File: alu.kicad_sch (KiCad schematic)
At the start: 20 parts, among them SW1 SW_DIP_x08

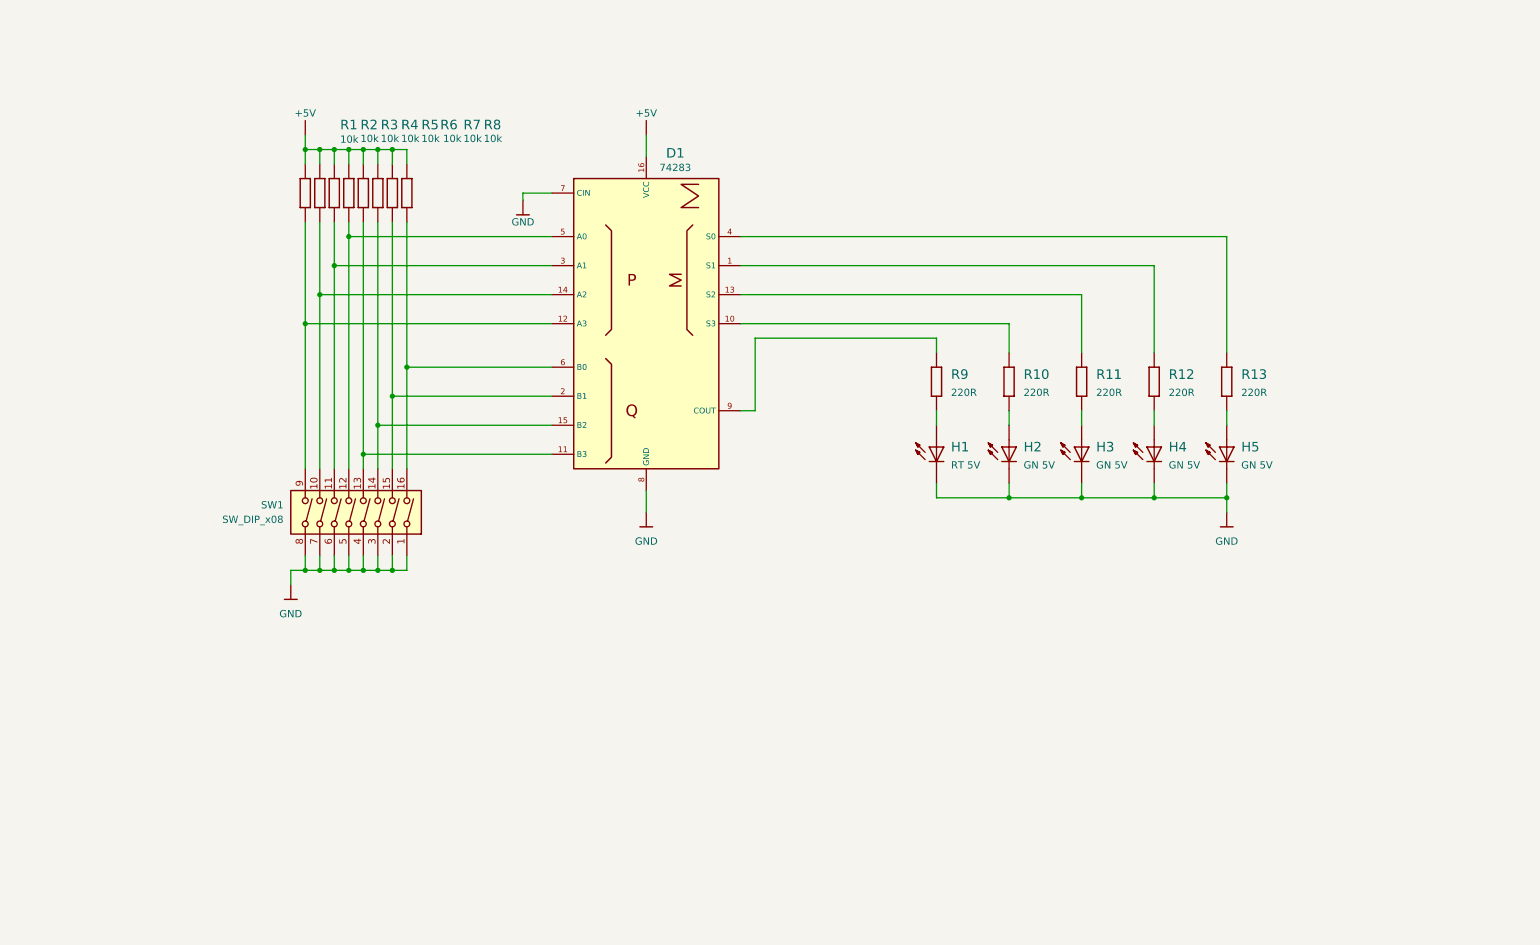
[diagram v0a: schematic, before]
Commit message: kys
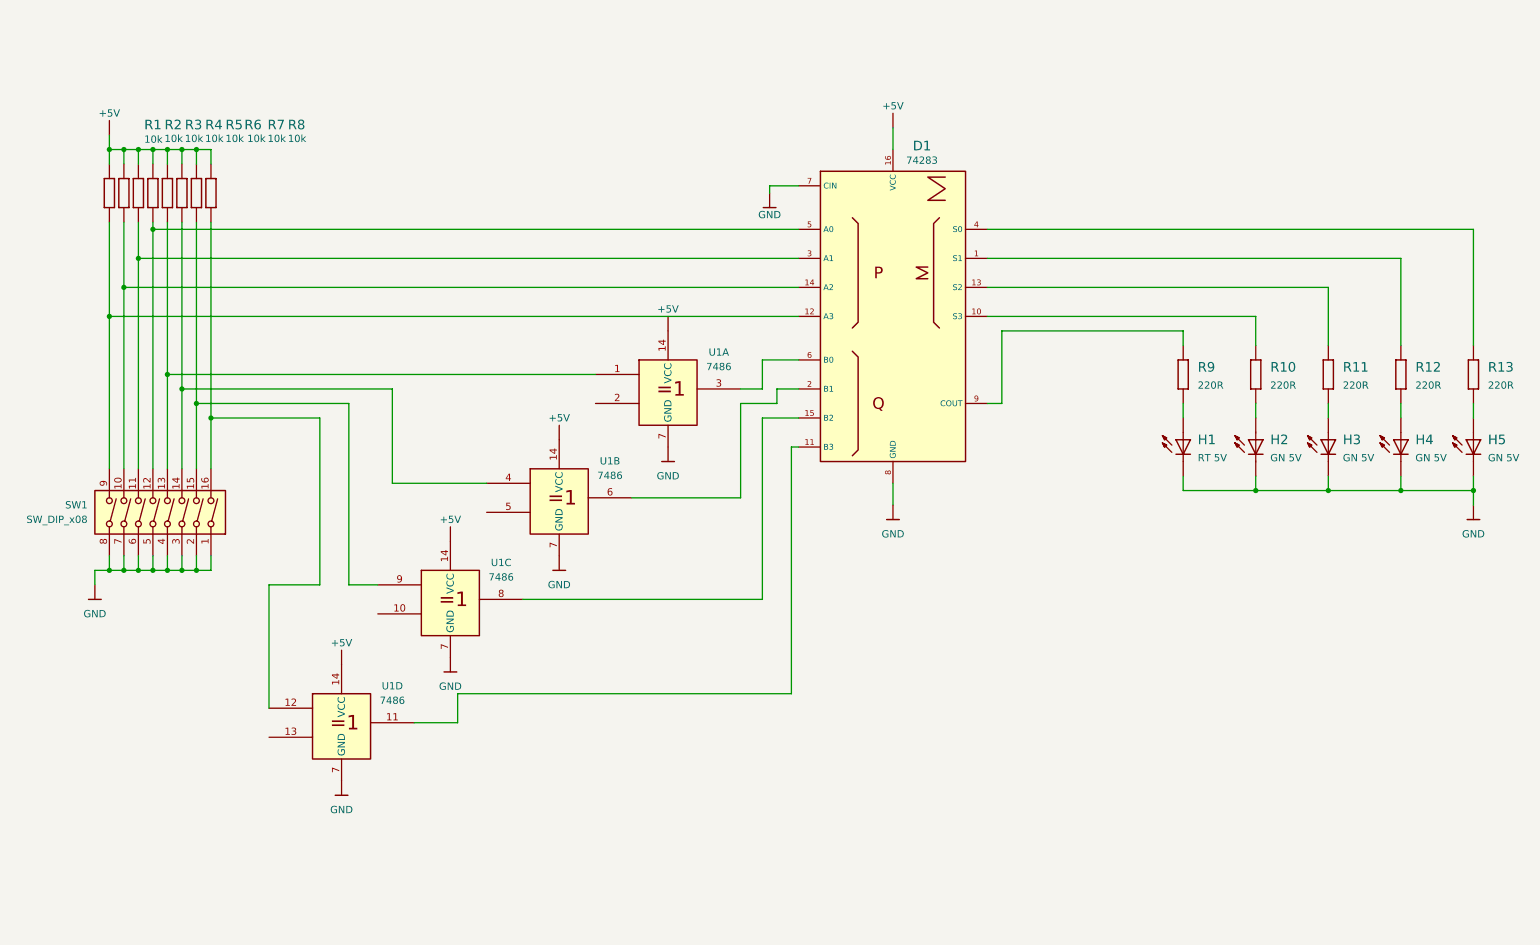
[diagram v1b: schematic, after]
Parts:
- added U1: 7486, symbol 74xx_IEEE:7486
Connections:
- net +5V: now also U1.14 (VCC), U1.14 (VCC), U1.14 (VCC), U1.14 (VCC)
- net GND: now also U1.7 (GND), U1.7 (GND), U1.7 (GND), U1.7 (GND)
- net at R5.1, SW1.13: now also U1.1; no longer D1.11 (B3)
- net at R6.1, SW1.14: now also U1.4; no longer D1.15 (B2)
- net at R7.1, SW1.15: now also U1.9; no longer D1.2 (B1)
- net at R8.1, SW1.16: now also U1.12; no longer D1.6 (B0)
- new net: D1.2 (B1), U1.6
- new net: D1.6 (B0), U1.3
- new net: D1.11 (B3), U1.11
- new net: D1.15 (B2), U1.8
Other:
- moved on the sheet: D1, H1, H2, H3, H4, H5, R1, R10, R11, R12, R13, R2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

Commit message: schem fixed
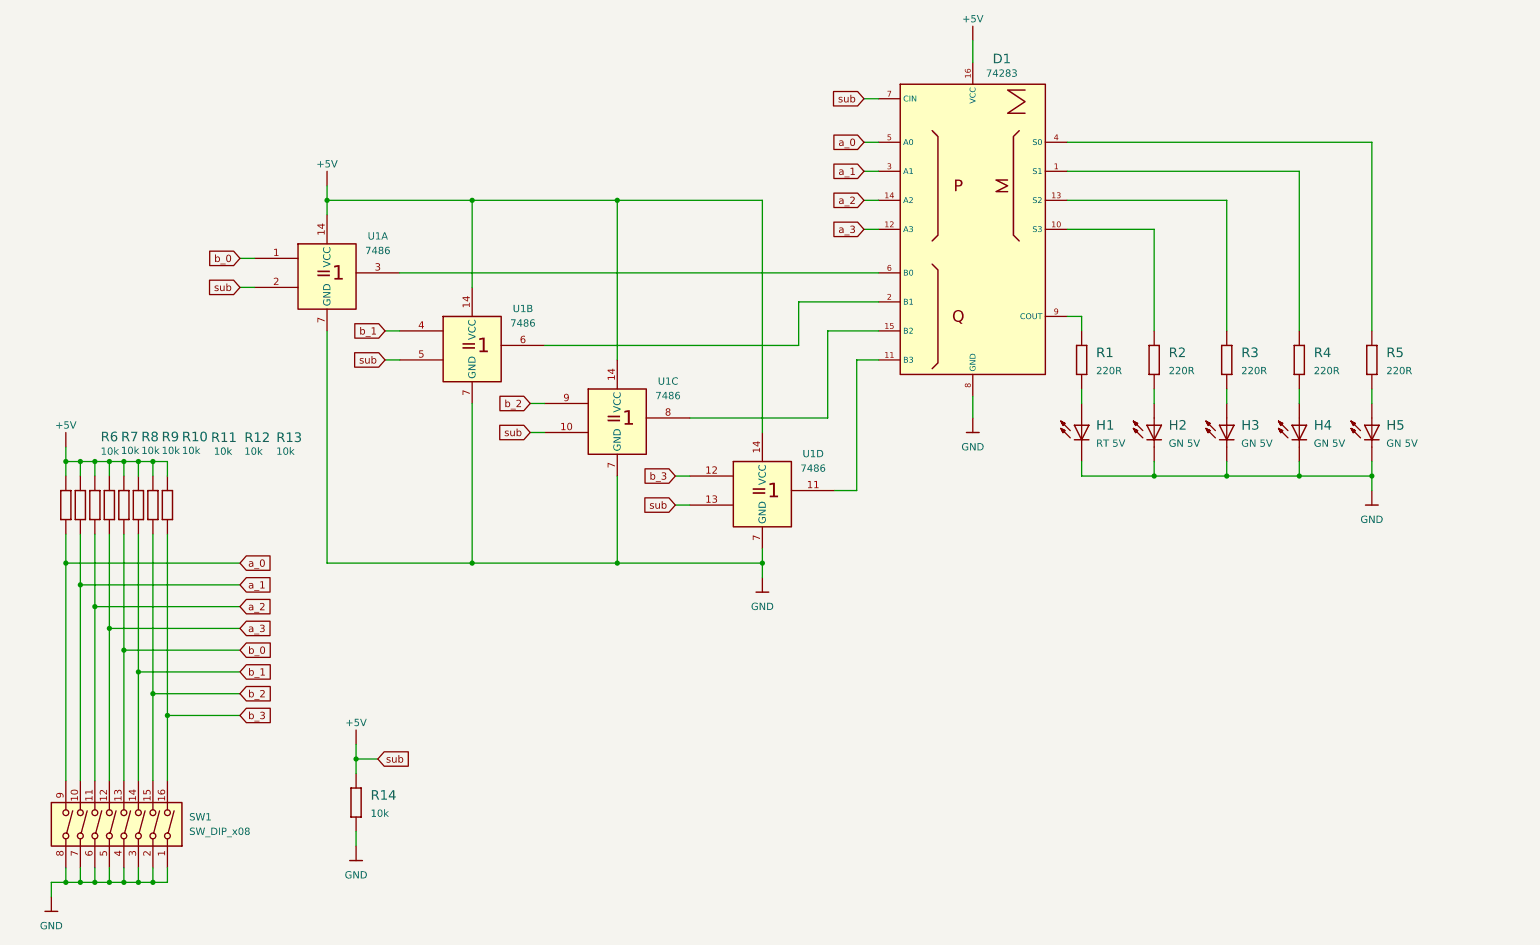
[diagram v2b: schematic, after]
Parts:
- added R14: 10k, ~footprint, symbol basic_AndF:R
- renumbered R9 to R1, R5 to R10, R6 to R11, R7 to R12, R8 to R13, R10 to R2, R11 to R3, R12 to R4, R13 to R5, R1 to R6, R2 to R7, R3 to R8, R4 to R9
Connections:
- net +5V: now also D1.7 (CIN), U1.10, U1.13, U1.2, U1.5, R14.2
- net GND: now also R14.1; no longer D1.7 (CIN)
- net a_1: now reaches R7.1, SW1.10
- net a_1: now also D1.3 (A1); no longer D1.14 (A2)
- net a_2: now reaches R8.1, SW1.11
- net a_2: now also D1.14 (A2); no longer D1.3 (A1)
- net a_3: now reaches R9.1, SW1.12
- net a_3: now also D1.12 (A3); no longer D1.5 (A0)
- net b_0: now reaches R10.1, SW1.13, U1.1
- net b_1: now reaches R11.1, SW1.14, U1.4
- net b_2: now reaches R12.1, SW1.15, U1.9
- net b_3: now reaches R13.1, SW1.16, U1.12
- net a_0: now reaches R6.1, SW1.9
- net a_0: now also D1.5 (A0); no longer D1.12 (A3)
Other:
- moved on the sheet: D1, H1, H2, H3, H4, H5, R1, R10, R11, R12, R13, R2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
